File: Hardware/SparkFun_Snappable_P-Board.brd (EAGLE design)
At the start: 129.5 x 66 mm, 128 parts

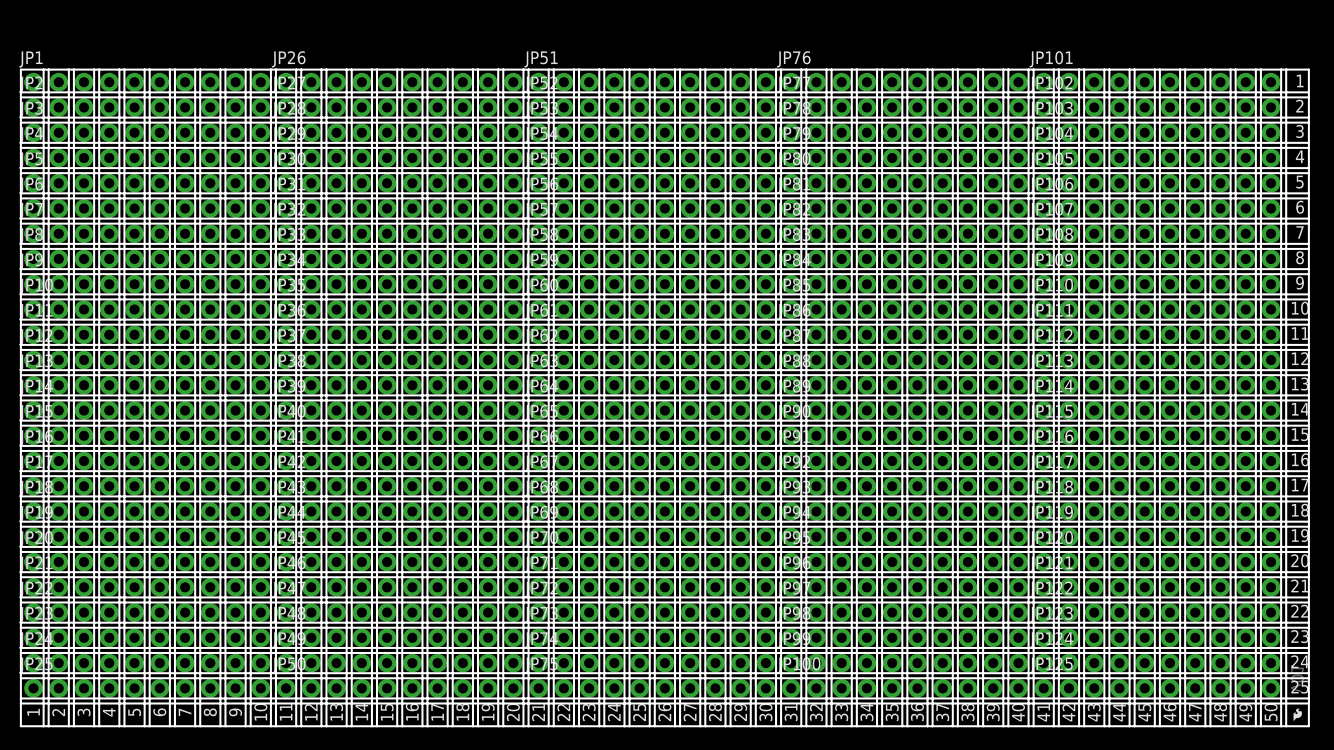
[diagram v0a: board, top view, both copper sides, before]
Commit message: Ready for protos
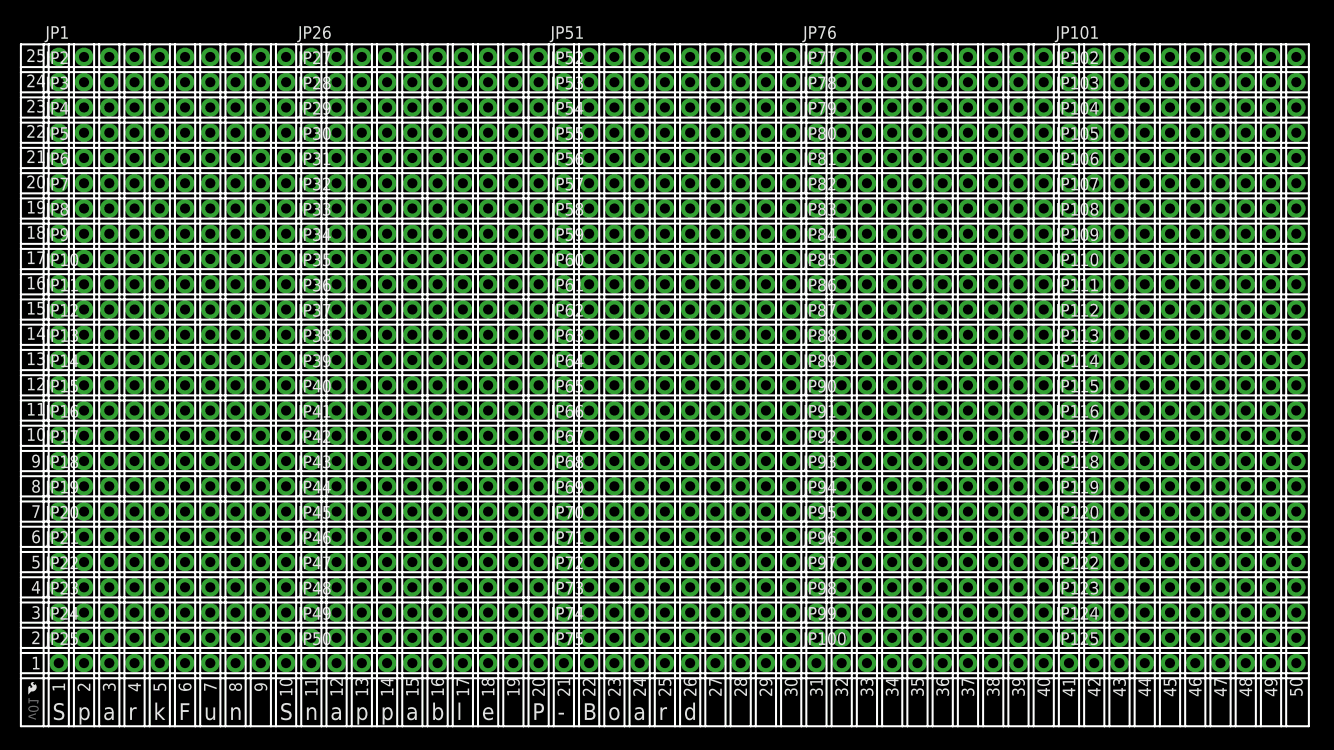
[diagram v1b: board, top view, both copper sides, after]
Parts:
- moved LOGO1 127.3 mm to (0.38, 0.13)
- moved LOGO2 127.3 mm to (1.91, 0.13)
- moved JP84 3.59 mm to (80.0, 44.5)
- moved JP91 3.59 mm to (80.0, 26.7)
- moved JP95 3.59 mm to (80.0, 16.5)
- moved JP96 3.59 mm to (80.0, 14.0)
- moved JP98 3.59 mm to (80.0, 8.89)
- moved JP100 3.59 mm to (80.0, 3.81)
- moved JP9 3.59 mm to (3.81, 44.5)
- moved JP34 3.59 mm to (29.2, 44.5)
- moved JP59 3.59 mm to (54.6, 44.5)
- moved JP76 3.59 mm to (80.0, 64.8)
- moved JP77 3.59 mm to (80.0, 62.2)
- moved JP78 3.59 mm to (80.0, 59.7)
- moved JP79 3.59 mm to (80.0, 57.1)
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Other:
- board size 129.5 x 66 mm -> 129.5 x 68.6 mm
- board text added: "-"
- board text added: "B"
- board text added: "F"
- board text added: "P"
- board text added: "S"
- board text added: "a"
- board text added: "b"
- board text added: "d"
- board text added: "e"
- board text added: "k"
- board text added: "l"
- board text added: "n"
- board text added: "o"
- board text added: "p"
- board text added: "r"
- board text added: "u"
- board text removed: "Snappable P-Board"
